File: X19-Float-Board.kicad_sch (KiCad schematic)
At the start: 2 parts

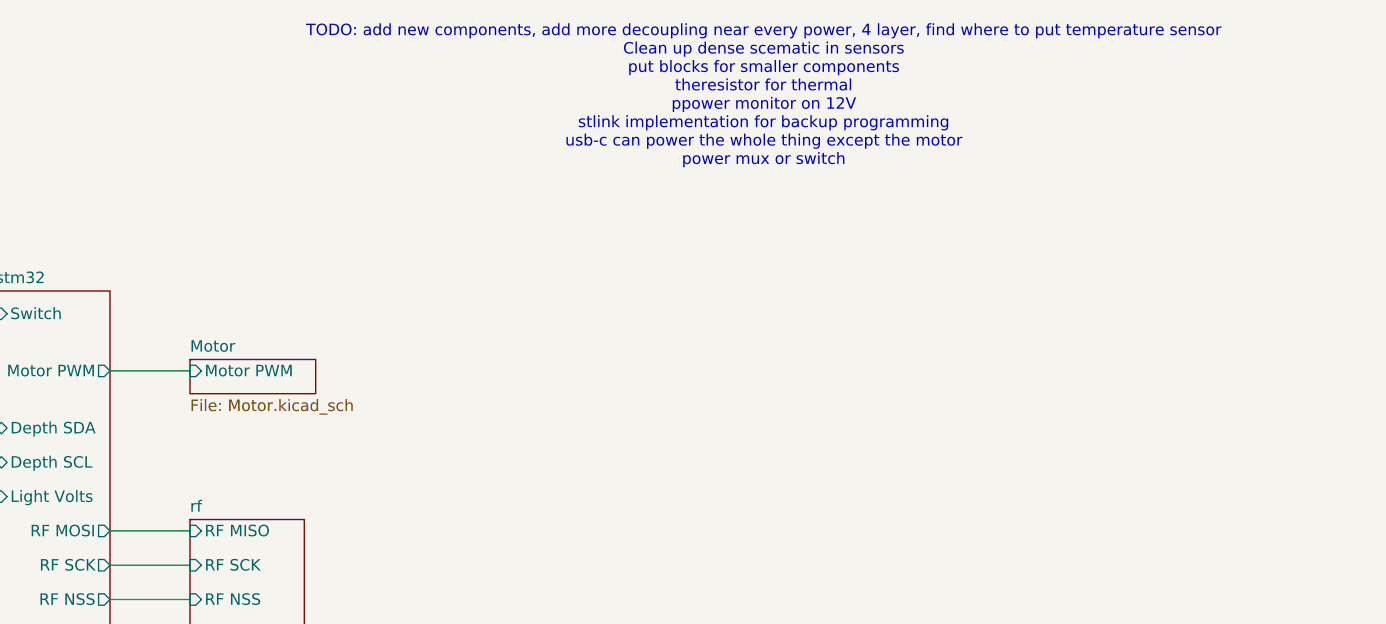
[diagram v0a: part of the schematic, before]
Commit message: Updated Schematic
Updated parts of todo list for schematic
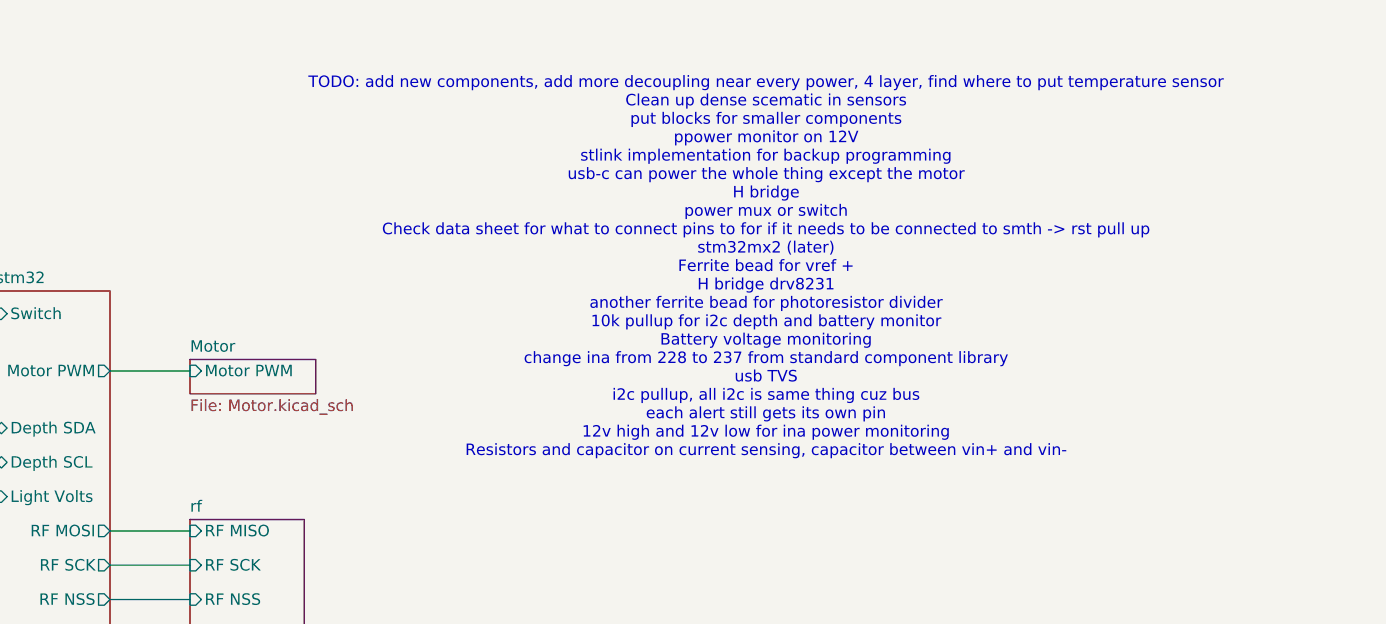
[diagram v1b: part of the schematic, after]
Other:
- note added: "TODO: add new components, add more decoupling near every power, 4 layer, find where to put temperature sensor Clean up dense scematic in sensors put blocks for smaller components ppower monitor on 12V stlink implementation for backup programming usb-c can power the whole thing except the motor H bridge power mux or switch Check data sheet for what to connect pins to for if it needs to be connecte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"
- note removed: "TODO: add new components, add more decoupling near every power, 4 layer, find where to put temperature sensor Clean up dense scematic in sensors put blocks for smaller components theresistor for thermal ppower monitor on 12V stlink implementation for backup programming usb-c can power the whole thing except the motor power mux or switch"
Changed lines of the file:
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@@
 		)
 	)
-	(text "TODO: add new components, add more decoupling near every power, 4 layer, find where to put temperature sensor\nClean up dense scematic in sensors\nput blocks for smaller components\ntheresistor for thermal\nppower monitor on 12V\nstlink implementation for backup programming\nusb-c can power the whole thing except the motor\npower mux or switch\n\n\n"
+	(text "TODO: add new components, add more decoupling near every power, 4 layer, find where to put temperature sensor\nClean up dense scematic in sensors\nput blocks for smaller components\nppower monitor on 12V\nstlink implementation for backup programming\nusb-c can power the whole thing except the motor\nH bridge\npower mux or switch\nCheck data sheet for what to connect pins to for if it needs to be connected to smth -> rst pull up \nstm32mx2 (later)\nFerrite bead for vref +\nH bridge drv8231\nanother ferrite bead for photoresistor divider\n10k pullup for i2c depth and battery monitor\nBattery voltage monitoring\nchange ina from 228 to 237 from standard component library\nusb TVS\ni2c pullup, all i2c is same thing cuz bus\neach alert still gets its own pin\n12v high and 12v low for ina power monitoring\nResistors and capacitor on current sensing, capacitor between vin+ and vin-\n\n\n"
 		(exclude_from_sim no)
-		(at 227.584 18.542 0)
+		(at 227.838 37.592 0)
 		(effects
 			(font
